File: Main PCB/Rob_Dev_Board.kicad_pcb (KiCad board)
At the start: 4 copper layers, 71 x 62.5 mm, 11 parts, among them J1 TYPE-C-31-M-12, J2 XT60PW-M, U1 DRV8245HQRXZRQ1, U2 ESP32-S3-WROOM-1U-N16R8, U3 DRV8245HQRXZRQ1, U4 PCA9685PW_118, U5 MPU-6050

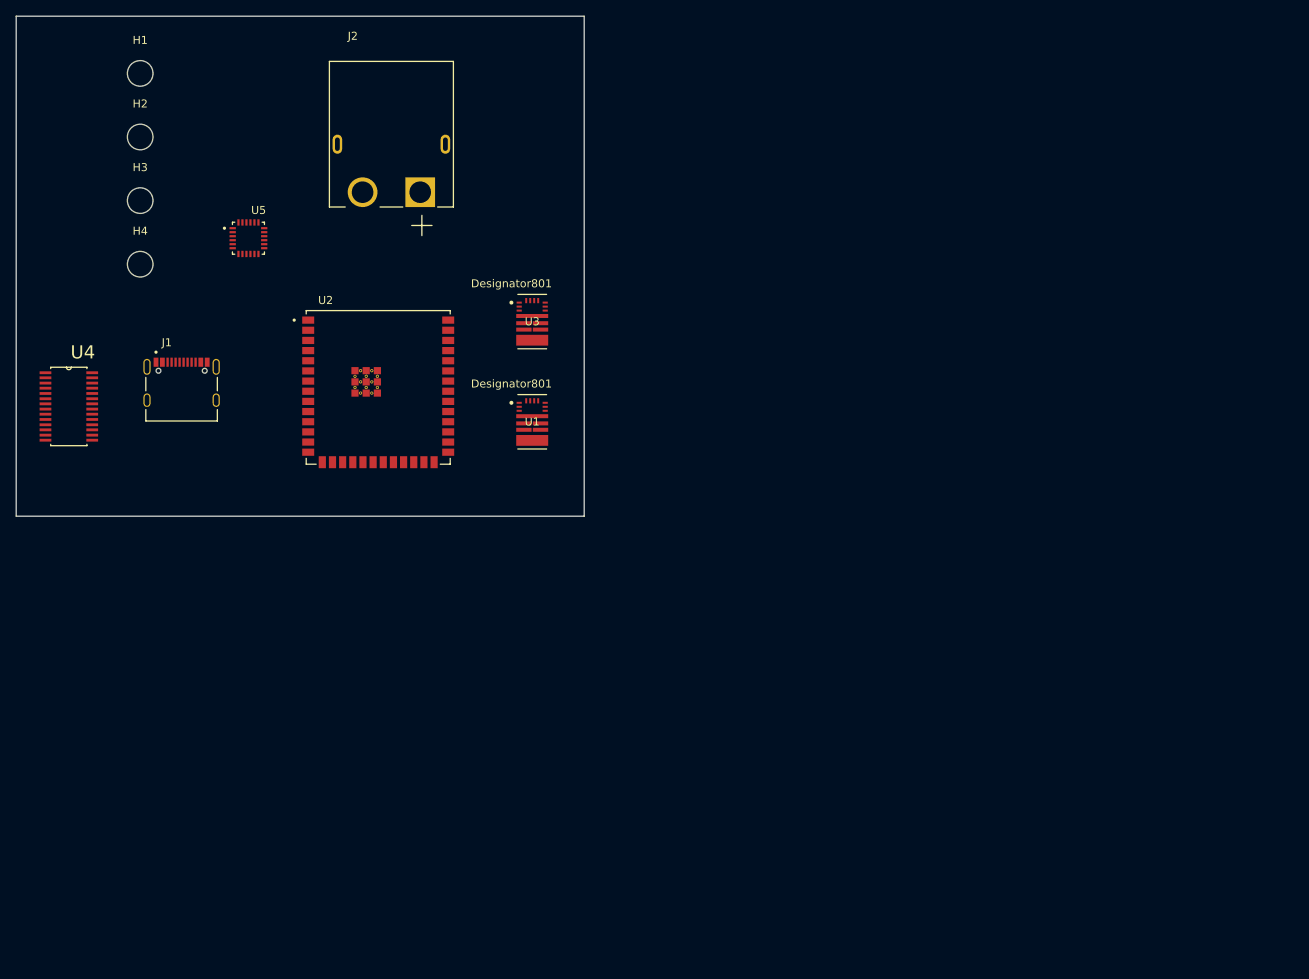
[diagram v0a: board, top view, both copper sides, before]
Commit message: Testing
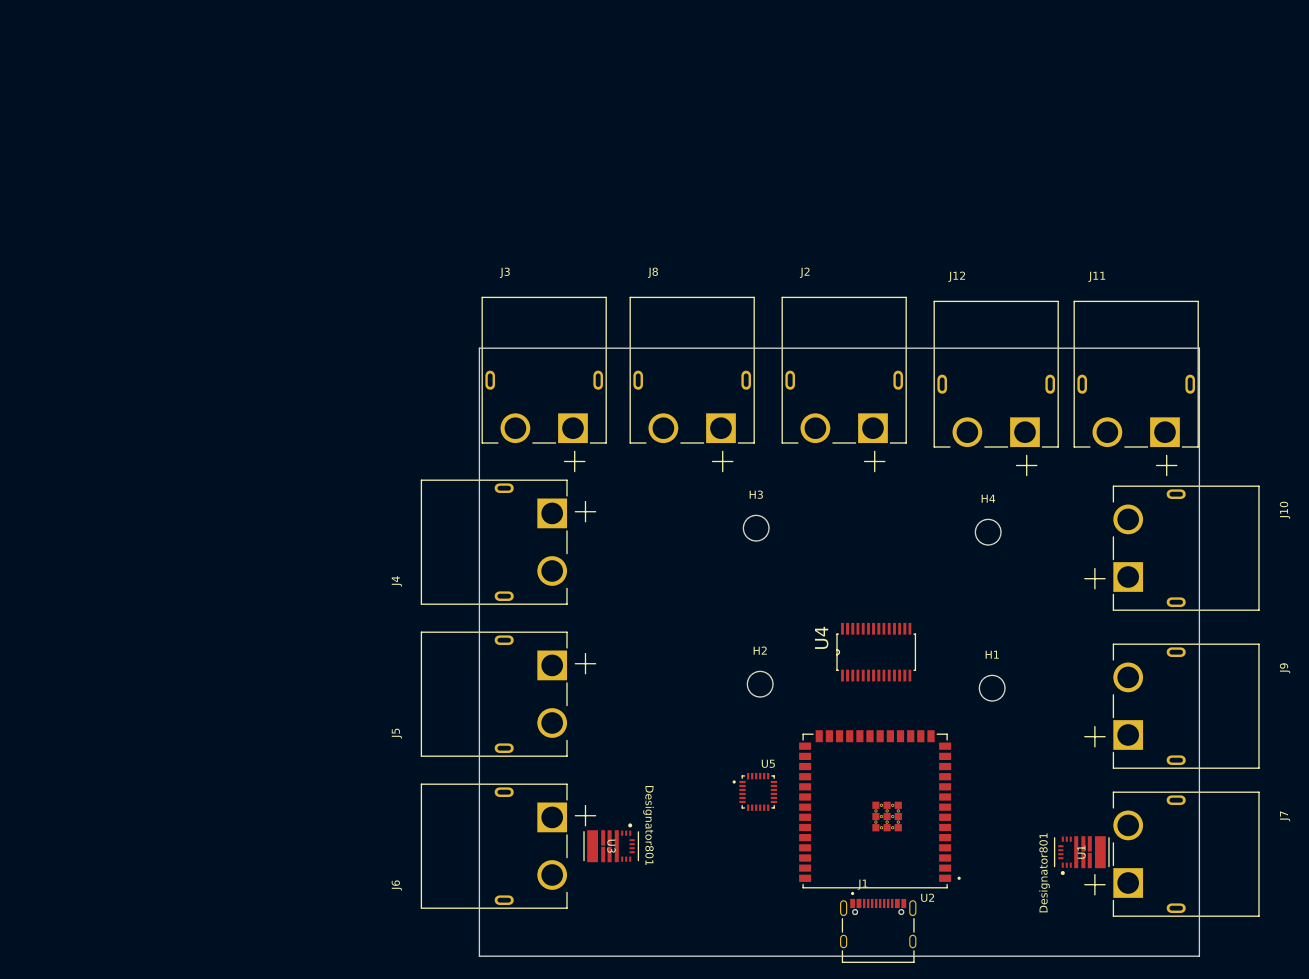
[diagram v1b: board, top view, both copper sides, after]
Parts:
- added J10: XT60PW-M, XT60PW-M Connector:AMASS_XT60PW-M, F.Cu at (184.0, 100.0)
- added J11: XT60PW-M, XT60PW-M Connector:AMASS_XT60PW-M, F.Cu at (179.0, 79.5)
- added J12: XT60PW-M, XT60PW-M Connector:AMASS_XT60PW-M, F.Cu at (161.5, 79.5)
- added J3: XT60PW-M, XT60PW-M Connector:AMASS_XT60PW-M, F.Cu at (105.0, 79.0)
- added J4: XT60PW-M, XT60PW-M Connector:AMASS_XT60PW-M, F.Cu at (100.0, 99.2)
- added J5: XT60PW-M, XT60PW-M Connector:AMASS_XT60PW-M, F.Cu at (100.0, 118.2)
- added J6: XT60PW-M, XT60PW-M Connector:AMASS_XT60PW-M, F.Cu at (100.0, 137.2)
- added J7: XT60PW-M, XT60PW-M Connector:AMASS_XT60PW-M, F.Cu at (184.0, 138.2)
- added J8: XT60PW-M, XT60PW-M Connector:AMASS_XT60PW-M, F.Cu at (123.5, 79.0)
- added J9: XT60PW-M, XT60PW-M Connector:AMASS_XT60PW-M, F.Cu at (184.0, 119.8)
- moved H1 131.3 mm to (161.0, 117.5)
- moved H4 111.2 mm to (160.5, 98.0)
- moved J1 110.3 mm to (146.8, 149.2)
- moved U4 105.5 mm to (146.5, 113.0), turned to 90 degrees
- moved H2 103.4 mm to (132.0, 117.0)
- moved U5 94.1 mm to (131.8, 130.5)
- moved U1 87.3 mm to (172.2, 138.0), turned to 90 degrees
- moved H3 87.2 mm to (131.5, 97.5)
- moved U2 81.6 mm to (146.4, 132.8), turned to 180 degrees
- moved U3 66.3 mm to (113.4, 137.2), turned to -90 degrees
- moved J2 63.8 mm to (142.5, 79.0)
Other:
- board size 71 x 62.5 mm -> 90 x 76 mm
